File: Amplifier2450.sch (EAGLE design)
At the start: 25 parts, among them IC1 7805DT, Q1 FDN360P, X1 SMA-142-0701-801/806, X2 SMA-142-0701-801/806

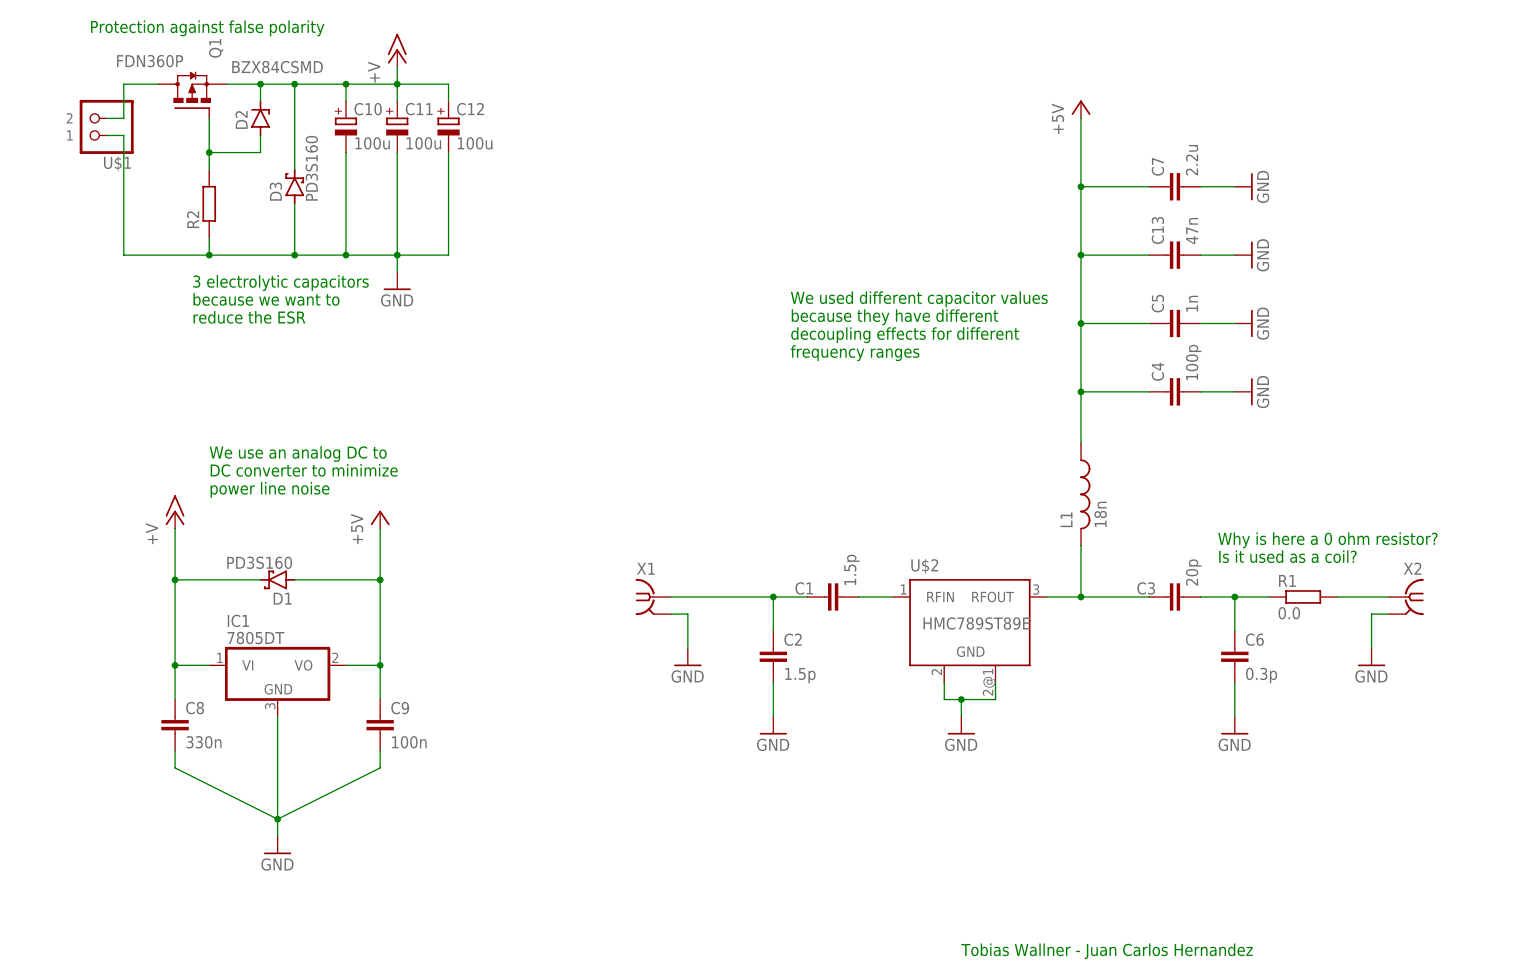
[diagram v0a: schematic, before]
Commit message: (Tobias): selected components and started the layout
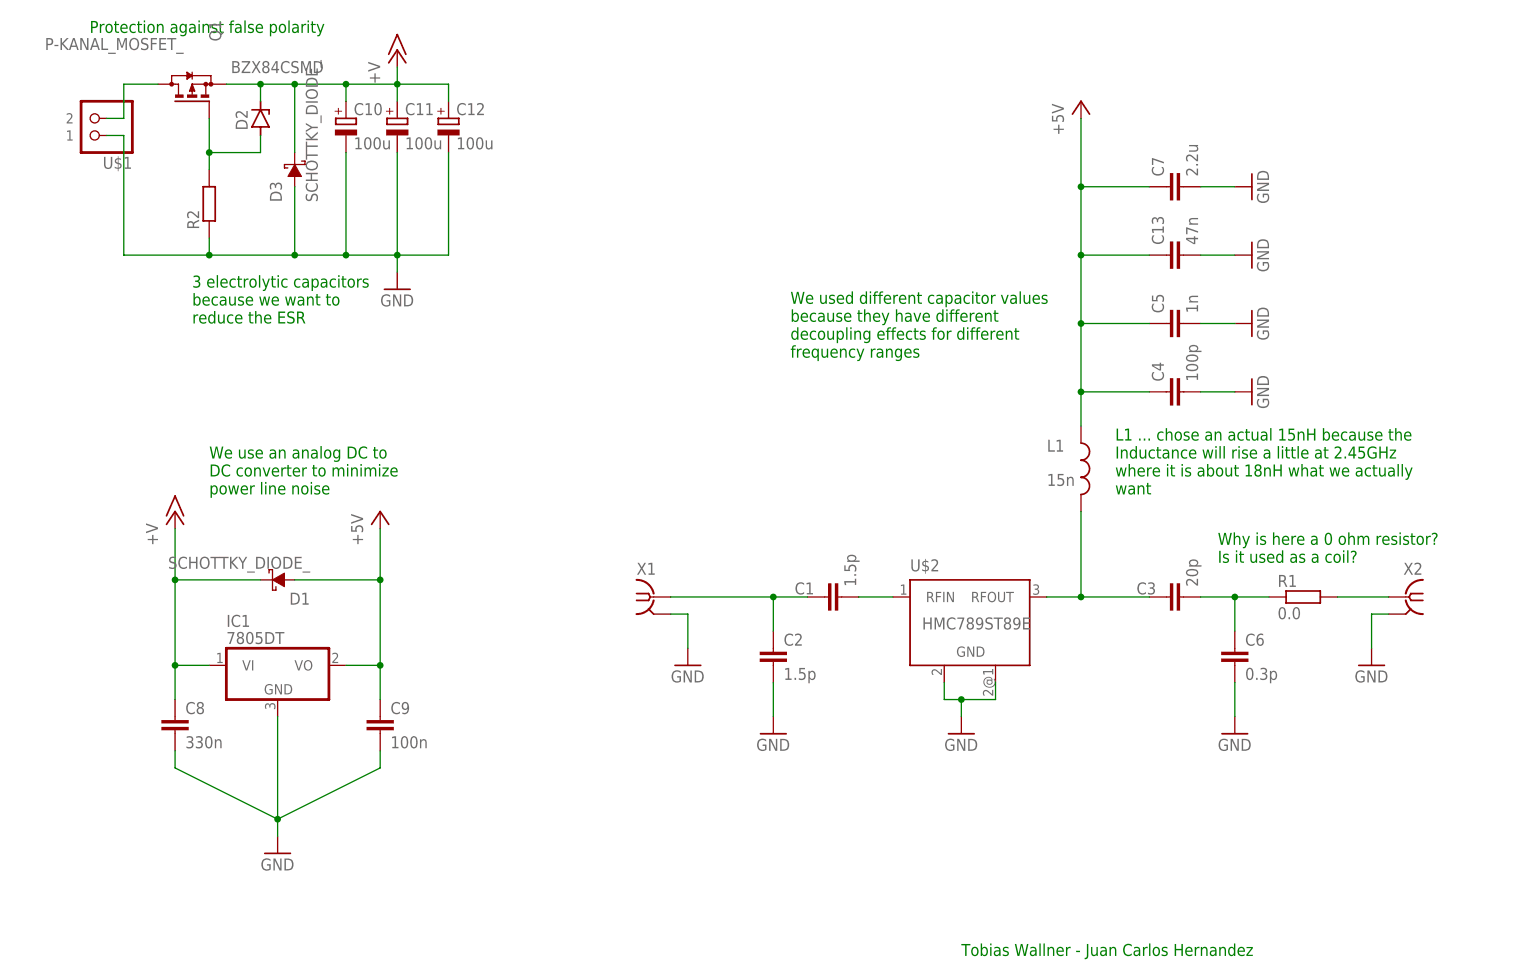
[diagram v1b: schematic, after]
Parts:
- D1, D3: value PD3S160 -> SCHOTTKY_DIODE_; device diode:PD3S160 -> own_htl3r-discrete-1:SCHOTTKY_DIODE_
- L1: value 18n -> 15n; device rcl:L-USL1812 -> own_htl3r-discrete-1:L_US_
- Q1: value FDN360P -> P-KANAL_MOSFET_; device transistor-power:FDN360P -> own_htl3r-discrete-1:P-KANAL_MOSFET_
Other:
- note added: "L1 ... chose an actual 15nH because the Inductance will rise a little at 2.45GHz where it is about 18nH what we actually want"
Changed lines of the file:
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@@
 <part name="P+2" library="supply1" library_urn="urn:adsk.eagle:library:371" deviceset="+15V" device="" value="+V"/>
 <part name="U$2" library="HMC789ST89E" deviceset="HMC789ST89E" device=""/>
-<part name="L1" library="rcl" library_urn="urn:adsk.eagle:library:334" deviceset="L-US" device="L1812" package3d_urn="urn:adsk.eagle:package:23494/2" value="18n"/>
+<part name="L1" library="own_htl3r-discrete-1" deviceset="L_US_" device="" value="15n"/>
 <part name="GND3" library="supply1" library_urn="urn:adsk.eagle:library:371" deviceset="GND" device=""/>
 <part name="GND4" library="supply1" library_urn="urn:adsk.eagle:library:371" deviceset="GND" device=""/>
@@
 <part name="GND10" library="supply1" library_urn="urn:adsk.eagle:library:371" deviceset="GND" device=""/>
 <part name="GND11" library="supply1" library_urn="urn:adsk.eagle:library:371" deviceset="GND" device=""/>
-<part name="D1" library="diode" library_urn="urn:adsk.eagle:library:210" deviceset="PD3S160" device="" package3d_urn="urn:adsk.eagle:package:43459/1"/>
-<part name="Q1" library="transistor-power" library_urn="urn:adsk.eagle:library:400" deviceset="FDN360P" device="" package3d_urn="urn:adsk.eagle:package:29529/2"/>
+<part name="D1" library="own_htl3r-discrete-1" deviceset="SCHOTTKY_DIODE_" device=""/>
+<part name="Q1" library="own_htl3r-discrete-1" deviceset="P-KANAL_MOSFET_" device=""/>
 <part name="R2" library="rcl" library_urn="urn:adsk.eagle:library:334" deviceset="R-EU_" device="R0805" package3d_urn="urn:adsk.eagle:package:23553/2"/>
 <part name="D2" library="diode" library_urn="urn:adsk.eagle:library:210" deviceset="BZX84CSMD" device="" package3d_urn="urn:adsk.eagle:package:43403/2"/>
 <part name="FRAME1" library="frames" library_urn="urn:adsk.eagle:library:229" deviceset="A4L-LOC" device=""/>
-<part name="D3" library="diode" library_urn="urn:adsk.eagle:library:210" deviceset="PD3S160" device="" package3d_urn="urn:adsk.eagle:package:43459/1"/>
+<part name="D3" library="own_htl3r-discrete-1" deviceset="SCHOTTKY_DIODE_" device=""/>
 </parts>
 <sheets>
@@
 <text x="35.56" y="149.86" size="1.778" layer="91" grouprefs="POWERINPUT">Protection against false polarity</text>
 <text x="165.1" y="12.7" size="1.778" layer="91">Tobias Wallner - Juan Carlos Hernandez</text>
+<text x="187.96" y="81.28" size="1.778" layer="91">L1 ... chose an actual 15nH because the
+Inductance will rise a little at 2.45GHz
+where it is about 18nH what we actually
+want</text>
 </plain>
 <instances>
@@
 <attribute name="VALUE" x="159.258" y="61.214" size="1.778" layer="96"/>
 </instance>
-<instance part="L1" gate="G$1" x="182.88" y="81.28" smashed="yes" grouprefs="AMPLIFIER">
-<attribute name="NAME" x="181.61" y="76.2" size="1.778" layer="95" rot="R90"/>
-<attribute name="VALUE" x="186.69" y="76.2" size="1.778" layer="96" rot="R90"/>
+<instance part="L1" gate="G$1" x="182.88" y="86.36" smashed="yes" rot="R270" grouprefs="AMPLIFIER">
+<attribute name="NAME" x="177.8" y="87.63" size="1.778" layer="95"/>
+<attribute name="VALUE" x="177.8" y="82.55" size="1.778" layer="96"/>
 </instance>
 <instance part="GND3" gate="1" x="205.74" y="45.72" smashed="yes" grouprefs="AMPLIFIER">
@@
 <attribute name="VALUE" x="223.52" y="53.34" size="1.778" layer="96"/>
 </instance>
-<instance part="D1" gate="G$1" x="63.5" y="68.58" smashed="yes" rot="R180" grouprefs="DC-DC_CONVERTER">
-<attribute name="NAME" x="65.786" y="66.675" size="1.778" layer="95" rot="R180"/>
-<attribute name="VALUE" x="65.786" y="72.009" size="1.778" layer="96" rot="R180"/>
-</instance>
-<instance part="Q1" gate="G$1" x="50.8" y="139.7" smashed="yes" rot="MR90" grouprefs="POWERINPUT">
-<attribute name="NAME" x="53.34" y="146.05" size="1.778" layer="95" rot="MR90"/>
-<attribute name="VALUE" x="49.53" y="144.78" size="1.778" layer="96" rot="MR0"/>
+<instance part="D1" gate="G$1" x="66.04" y="68.58" smashed="yes" rot="R180" grouprefs="DC-DC_CONVERTER">
+<attribute name="NAME" x="68.326" y="66.675" size="1.778" layer="95" rot="R180"/>
+<attribute name="VALUE" x="68.326" y="72.009" size="1.778" layer="96" rot="R180"/>
+</instance>
+<instance part="Q1" gate="G$1" x="50.8" y="142.24" smashed="yes" rot="MR90" grouprefs="POWERINPUT">
+<attribute name="NAME" x="53.34" y="148.59" size="1.778" layer="95" rot="MR90"/>
+<attribute name="VALUE" x="49.53" y="147.32" size="1.778" layer="96" rot="MR0"/>
 </instance>
 <instance part="R2" gate="G$1" x="53.34" y="124.46" smashed="yes" rot="R90" grouprefs="POWERINPUT">
@@
 <junction x="53.34" y="116.84" grouprefs="POWERINPUT"/>
 <pinref part="D3" gate="G$1" pin="A"/>
-<wire x1="66.04" y1="124.46" x2="66.04" y2="116.84" width="0.1524" layer="91"/>
+<wire x1="66.04" y1="127" x2="66.04" y2="116.84" width="0.1524" layer="91"/>
 <junction x="66.04" y="116.84"/>
 </segment>
@@
 <junction x="60.96" y="142.24" grouprefs="POWERINPUT"/>
 <pinref part="D3" gate="G$1" pin="C"/>
-<wire x1="66.04" y1="129.54" x2="66.04" y2="142.24" width="0.1524" layer="91"/>
+<wire x1="66.04" y1="132.08" x2="66.04" y2="142.24" width="0.1524" layer="91"/>
 <junction x="66.04" y="142.24"/>
 </segment>
@@
 <pinref part="L1" gate="G$1" pin="1"/>
 <pinref part="C4" gate="G$1" pin="1"/>
-<wire x1="182.88" y1="88.9" x2="182.88" y2="96.52" width="0.1524" layer="91" grouprefs="AMPLIFIER"/>
+<wire x1="182.88" y1="91.44" x2="182.88" y2="96.52" width="0.1524" layer="91" grouprefs="AMPLIFIER"/>
 <wire x1="182.88" y1="96.52" x2="193.04" y2="96.52" width="0.1524" layer="91" grouprefs="AMPLIFIER"/>
 <pinref part="C5" gate="G$1" pin="1"/>
@@
 <wire x1="177.8" y1="66.04" x2="182.88" y2="66.04" width="0.1524" layer="91" grouprefs="AMPLIFIER"/>
 <pinref part="L1" gate="G$1" pin="2"/>
-<wire x1="182.88" y1="73.66" x2="182.88" y2="66.04" width="0.1524" layer="91" grouprefs="AMPLIFIER"/>
+<wire x1="182.88" y1="78.74" x2="182.88" y2="66.04" width="0.1524" layer="91" grouprefs="AMPLIFIER"/>
 <pinref part="C3" gate="G$1" pin="1"/>
 <wire x1="182.88" y1="66.04" x2="193.04" y2="66.04" width="0.1524" layer="91" grouprefs="AMPLIFIER"/>
